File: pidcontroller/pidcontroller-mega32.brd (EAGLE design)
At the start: 100 x 75.4 mm, 30 parts, among them IC2 MAX3232CWE, IC3 MEGA32-A

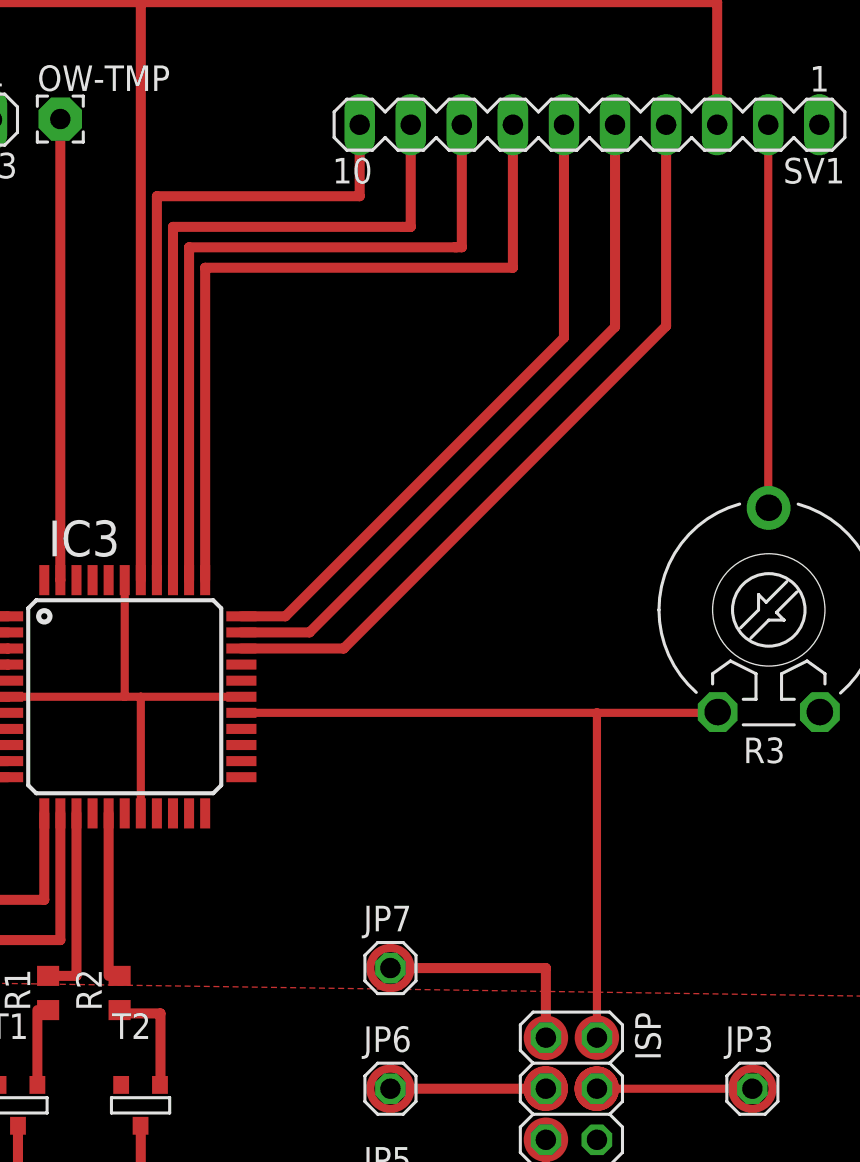
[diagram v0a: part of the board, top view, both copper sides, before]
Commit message: updated
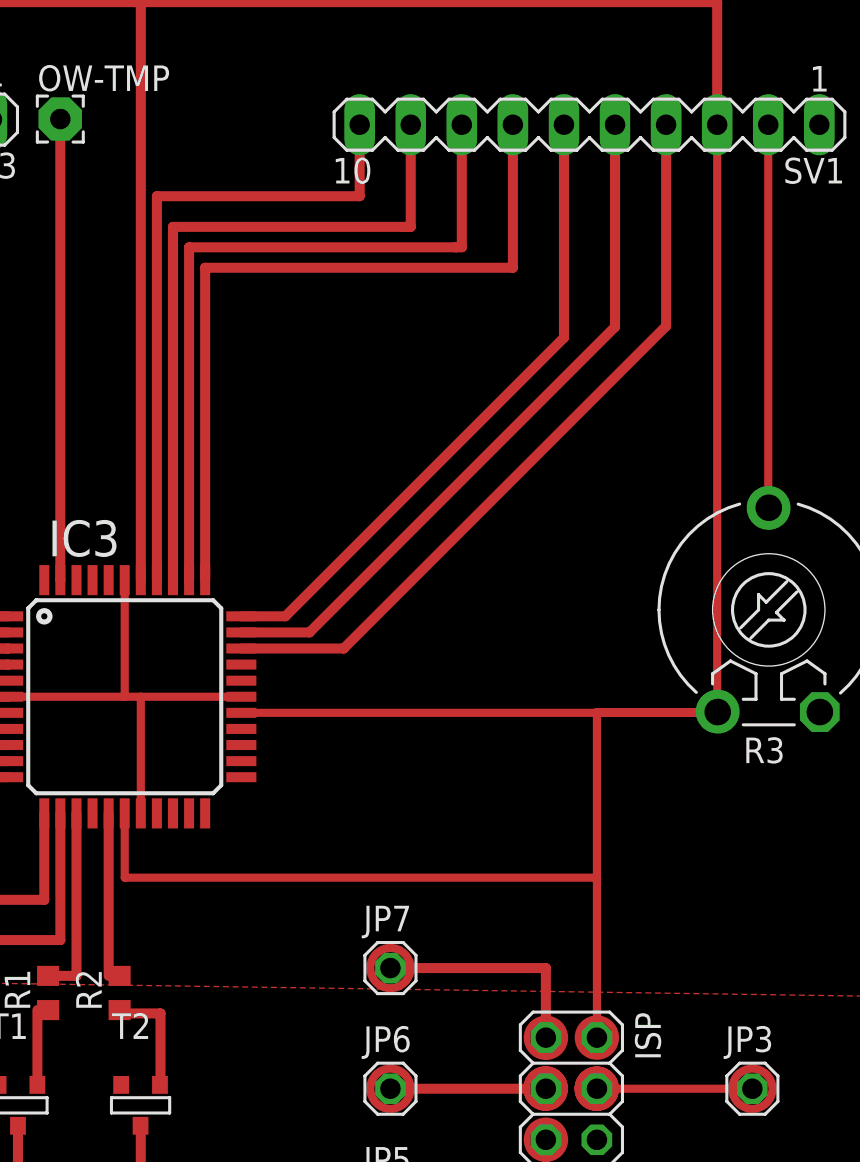
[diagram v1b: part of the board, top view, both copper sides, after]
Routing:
- net VCC: track 236.6 -> 298.6 mm
